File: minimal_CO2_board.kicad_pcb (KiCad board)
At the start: 2 copper layers, 1 part, among them U1 ESP32-C3_SUPERMINI

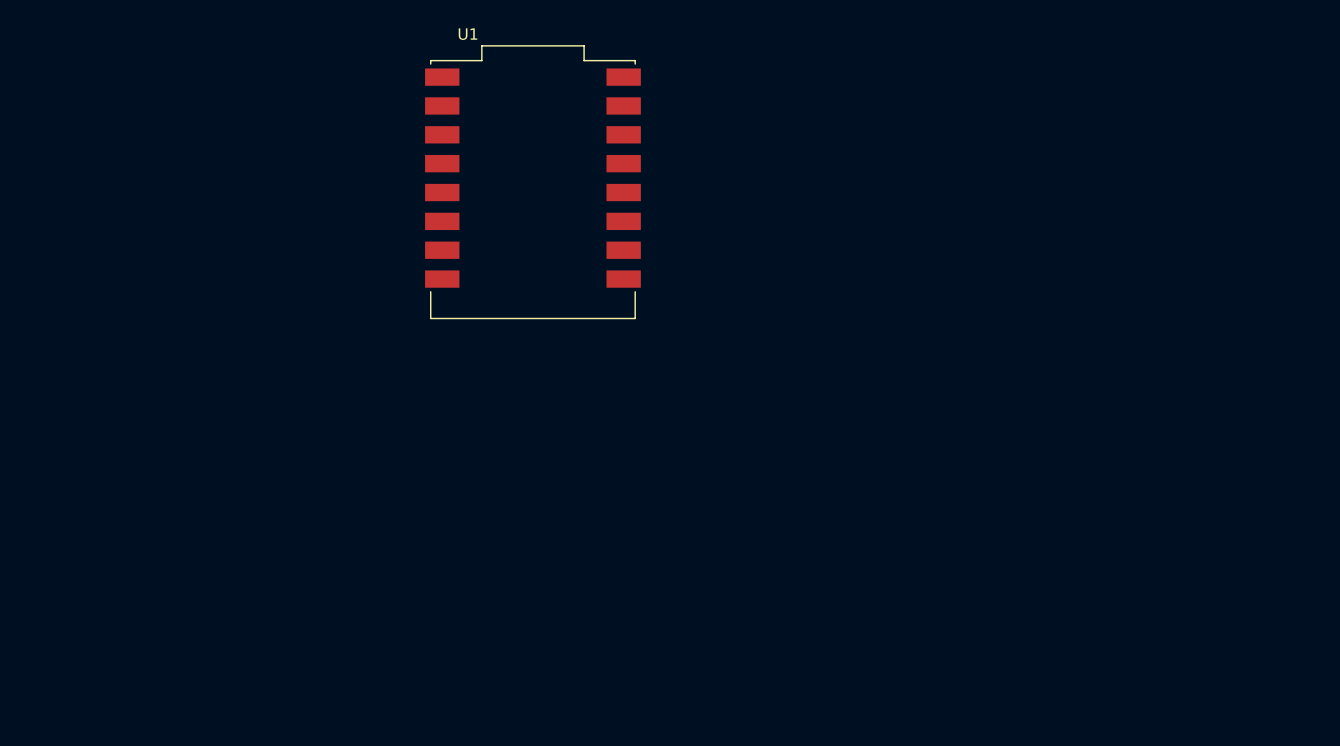
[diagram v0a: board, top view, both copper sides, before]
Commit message: changes
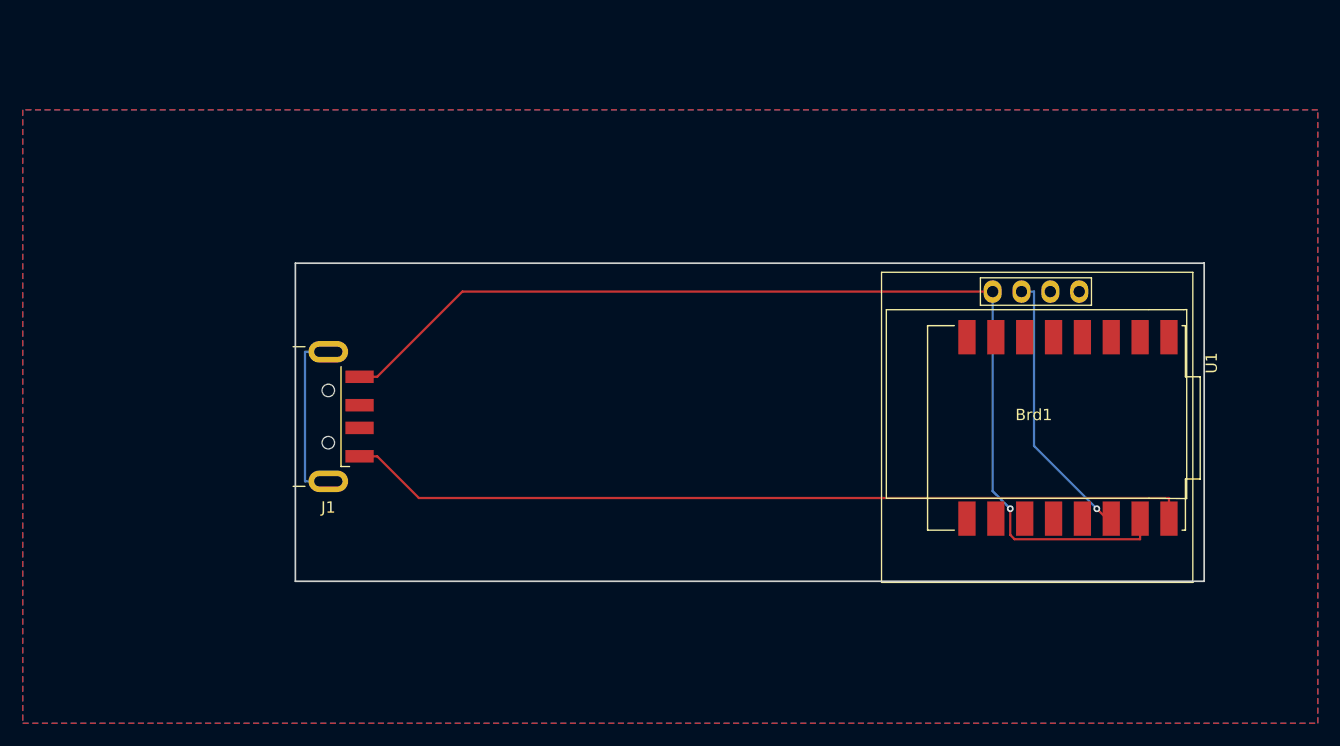
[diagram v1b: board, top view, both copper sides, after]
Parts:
- added Brd1: SSD1306, CustomLibrary:128x64OLED, F.Cu at (125.0, 100.6)
- added J1: USB_A, Connector_USB:USB_A_CNCTech_1001-011-01101_Horizontal, F.Cu at (56.0, 101.0)
- moved U1 50.6 mm to (127.0, 102.0), turned to -90 degrees
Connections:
- U1 pad 3.3: unconnected-(U1-3V3-Pad3.3) -> +3.3V
- U1 pad 5V: unconnected-(U1-Pad5V) -> +5V
- U1 pad G: unconnected-(U1-GND-PadG) -> GND
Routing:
- net GND: track 0.00 -> 94.3 mm, vias 0 -> 1
- net +5V: track 0.00 -> 74.6 mm
- net +3.3V: track 0.00 -> 24.1 mm, vias 0 -> 1
- net unconnected-(J1-Shield-Pad5): track 0.00 -> 15.5 mm
- added copper zone on B.Cu, net (none)
- added copper zone on F.Cu, net (none)
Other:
- board outline added: 80 x 28 mm
